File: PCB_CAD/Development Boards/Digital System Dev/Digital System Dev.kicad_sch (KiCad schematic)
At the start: 43 parts, among them J1 STLINK, J2 FADER, J7 SPI_MASTER, SW1 RESET, U1 STM32G474VETx, X1 HSE_24

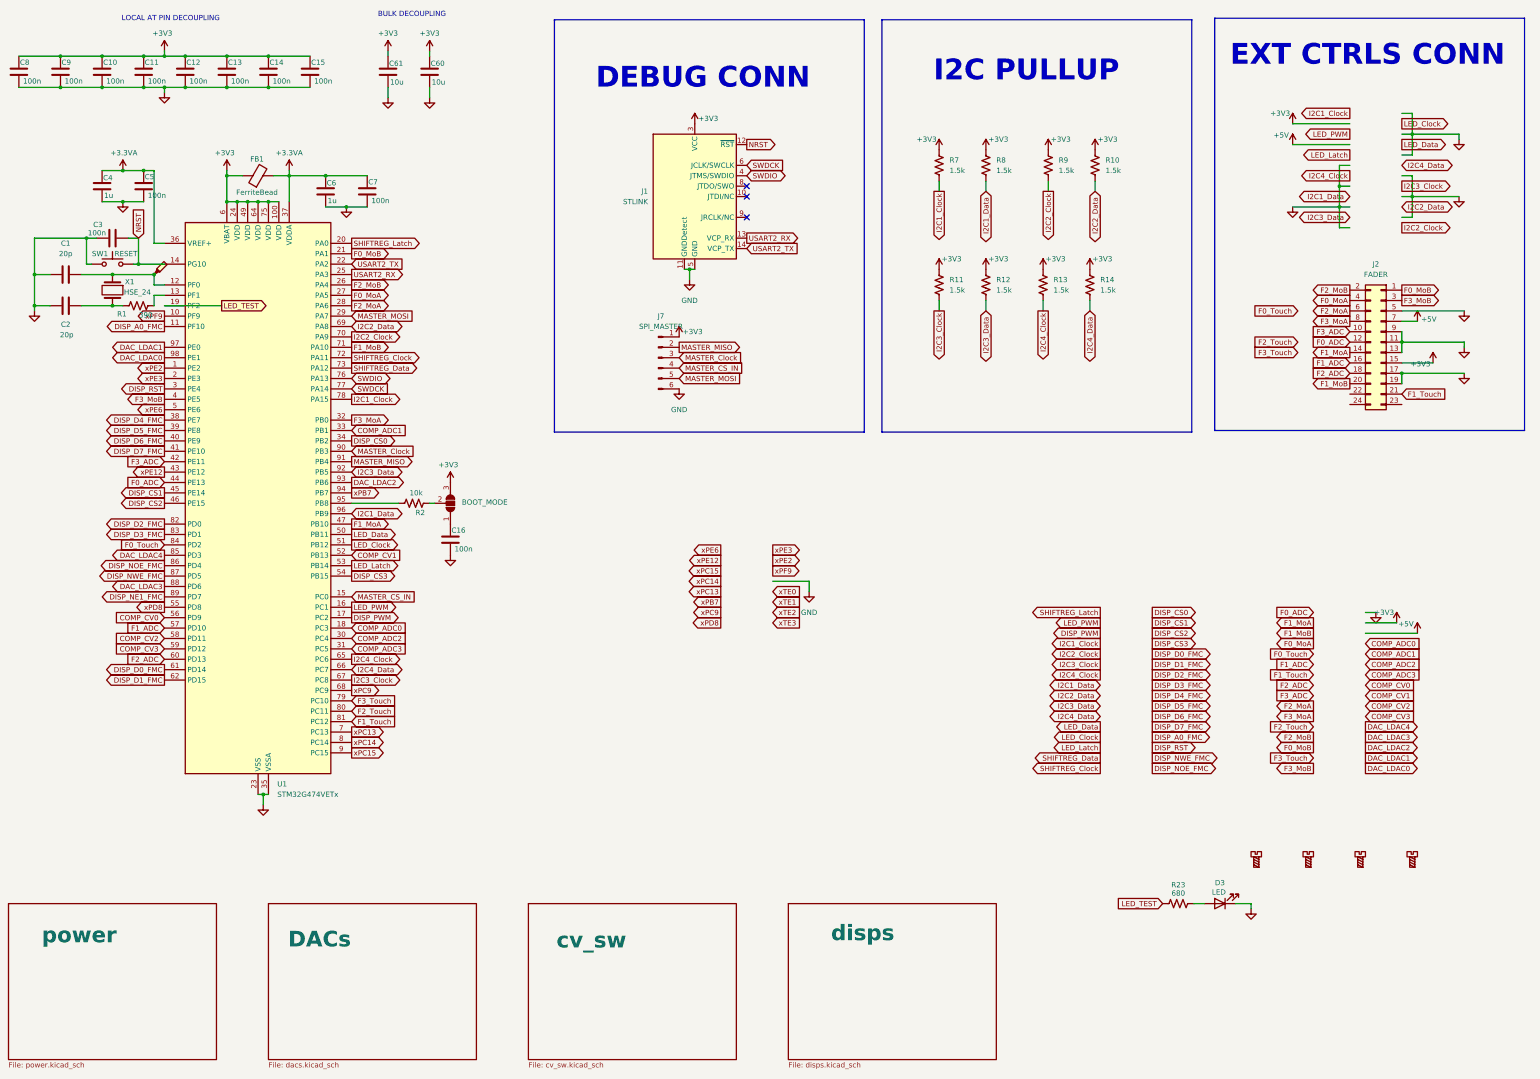
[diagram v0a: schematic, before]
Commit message: digital dev (or maybe final) board
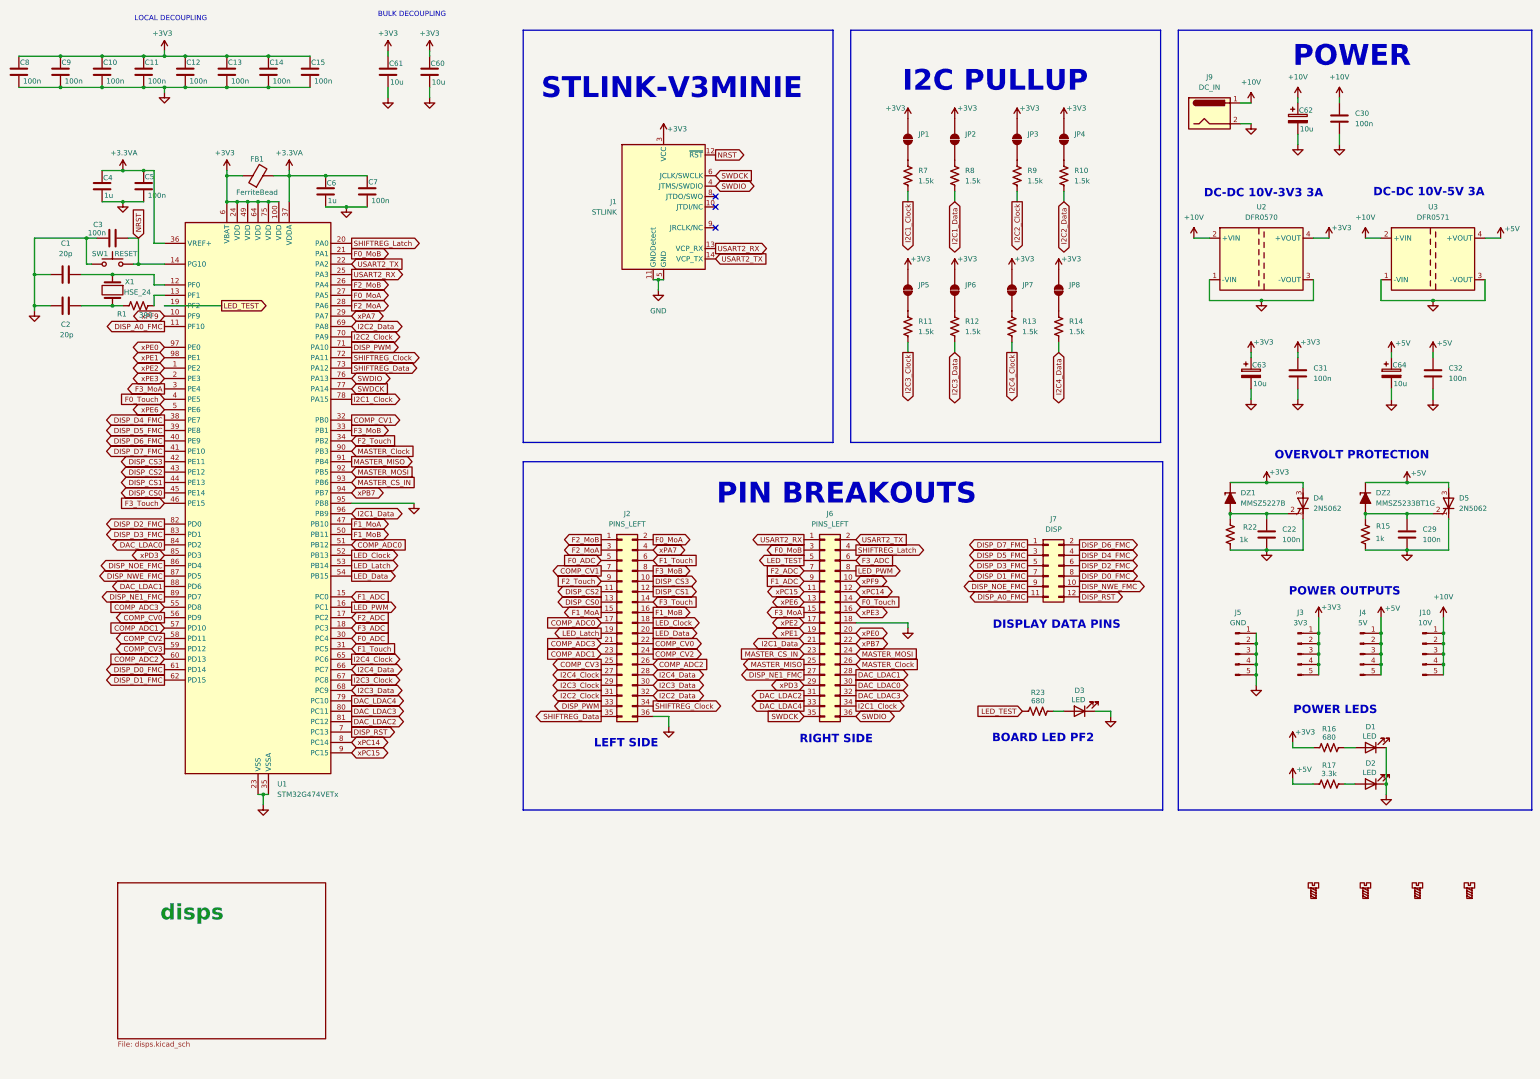
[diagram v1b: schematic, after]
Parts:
- removed C16: 100n, Capacitor_SMD:C_0603_1608Metric, symbol Device:C
- removed J2: FADER, Connector_PinHeader_1.27mm:PinHeader_2x12_P1.27mm_Vertical, symbol Connector_Generic:Conn_02x12_Odd_Even
- removed J7: SPI_MASTER, Connector_PinHeader_2.54mm:PinHeader_1x06_P2.54mm_Vertical, symbol Connector:Conn_01x06_Pin
- removed R2: 10k, Resistor_SMD:R_0603_1608Metric, symbol Device:R_US
- removed SP1: BOOT_MODE, Jumper:SolderJumper-3_P2.0mm_Open_TrianglePad1.0x1.5mm, symbol Jumper:SolderJumper_3_Open
- removed TP11: TestPoint_Probe, TestPoint:TestPoint_Keystone_5019_Miniature, symbol Connector:TestPoint_Probe
- added C22, C29, C30, C31, C32: 100n, Capacitor_SMD:C_0603_1608Metric, symbol Device:C
- added C62, C63, C64: 10u, Capacitor_SMD:CP_Elec_6.3x5.8, symbol Device:C_Polarized
- added D1, D2: LED, LED_SMD:LED_0603_1608Metric, symbol Device:LED
- added D4, D5: 2N5062, Package_TO_SOT_THT:TO-92, symbol Device:Q_SCR_KGA
- added DZ1: MMSZ5227B, Diode_SMD:D_SOD-123, symbol PCM_Diode_Zener_AKL:D_Zener_Generic
- added DZ2: MMSZ5233BT1G, Diode_SMD:D_SOD-123, symbol PCM_Diode_Zener_AKL:D_Zener_Generic
- added J10: 10V, Connector_PinSocket_2.54mm:PinSocket_1x05_P2.54mm_Vertical, symbol Connector:Conn_01x05_Pin
- added J2, J6: PINS_LEFT, Connector_PinHeader_2.54mm:PinHeader_2x18_P2.54mm_Vertical, symbol Connector_Generic:Conn_02x18_Odd_Even
- added J3: 3V3, Connector_PinSocket_2.54mm:PinSocket_1x05_P2.54mm_Vertical, symbol Connector:Conn_01x05_Pin
- added J4: 5V, Connector_PinSocket_2.54mm:PinSocket_1x05_P2.54mm_Vertical, symbol Connector:Conn_01x05_Pin
- added J5: GND, Connector_PinSocket_2.54mm:PinSocket_1x05_P2.54mm_Vertical, symbol Connector:Conn_01x05_Pin
- added J7: DISP, Connector_PinHeader_2.54mm:PinHeader_2x06_P2.54mm_Vertical, symbol Connector_Generic:Conn_02x06_Odd_Even
- added J9: DC_IN, Connector_BarrelJack:BarrelJack_Horizontal, symbol Connector:Barrel_Jack
- added JP1, JP2, JP3, JP4, JP5, JP6, JP7, JP8: SolderJumper_2_Open, Jumper:SolderJumper-2_P1.3mm_Open_TrianglePad1.0x1.5mm, symbol Jumper:SolderJumper_2_Open
- added R15, R22: 1k, Resistor_SMD:R_0603_1608Metric, symbol Device:R_US
- added R16: 680, Resistor_SMD:R_0603_1608Metric, symbol Device:R_US
- added R17: 3.3k, Resistor_SMD:R_0603_1608Metric, symbol Device:R_US
- added U2: DFR0570, My Footprints:DFR05xx_DC-DC, symbol Regulator_Switching:CRE1S0305S3C
- added U3: DFR0571, My Footprints:DFR05xx_DC-DC, symbol Regulator_Switching:CRE1S0305S3C
- H1, H2, H3, H4: LCSC (none) -> DNP
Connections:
- net xPC13 is gone; now on net DISP_RST: U1.7 (PC13)
- net xPC9 is gone; now on net I2C3_Data: U1.68 (PC9)
- net xPD8 is gone; now on net COMP_ADC3: U1.55 (PD8)
- net xPE12 is gone; now on net DISP_CS2: U1.43 (PE12)
- net +3V3: now also C31.1, C63.1, D4.3 (A), DZ1.1 (K), J3.1 (Pin_1), J3.2 (Pin_2), J3.3 (Pin_3), J3.4 (Pin_4), J3.5 (Pin_5), JP1.2 (B), JP2.2 (B), JP3.2 (B), JP4.2 (B), JP5.2 (B), JP6.2 (B), JP7.2 (B), JP8.2 (B), R16.1, U2.4 (+VOUT); no longer R10.1, R11.1, R12.1, R13.1, R14.1, R7.1, R8.1, R9.1
- net +5V: now also C32.1, C64.1, D5.3 (A), DZ2.1 (K), J4.1 (Pin_1), J4.2 (Pin_2), J4.3 (Pin_3), J4.4 (Pin_4), J4.5 (Pin_5), R17.1, U3.4 (+VOUT)
- net COMP_ADC0: now also U1.51 (PB12), J2.17 (Pin_17); no longer U1.18 (PC3)
- net COMP_ADC1: now also U1.57 (PD10), J2.23 (Pin_23); no longer U1.33 (PB1)
- net COMP_ADC2: now also U1.60 (PD13), J2.26 (Pin_26); no longer U1.30 (PC4)
- net COMP_ADC3: now also J2.21 (Pin_21); no longer U1.31 (PC5)
- net COMP_CV0: now also J2.22 (Pin_22)
- net COMP_CV1: now also U1.32 (PB0), J2.7 (Pin_7); no longer U1.52 (PB13)
- net COMP_CV2: now also J2.24 (Pin_24)
- net COMP_CV3: now also J2.25 (Pin_25)
- net DAC_LDAC0: now also U1.84 (PD2), J6.30 (Pin_30); no longer U1.98 (PE1)
- net DAC_LDAC1: now also U1.88 (PD6), J6.28 (Pin_28); no longer U1.97 (PE0)
- net DAC_LDAC2: now also U1.81 (PC12), J6.31 (Pin_31); no longer U1.93 (PB6)
- net DAC_LDAC3: now also U1.80 (PC11), J6.32 (Pin_32); no longer U1.88 (PD6)
- net DAC_LDAC4: now also U1.79 (PC10), J6.33 (Pin_33); no longer U1.85 (PD3)
- net DISP_A0_FMC: now also J7.11 (Pin_11)
- net DISP_CS0: now also U1.45 (PE14), J2.13 (Pin_13); no longer U1.34 (PB2)
- net DISP_CS1: now also U1.44 (PE13), J2.12 (Pin_12); no longer U1.45 (PE14)
- net DISP_CS2: now also J2.11 (Pin_11); no longer U1.46 (PE15)
- net DISP_CS3: now also U1.42 (PE11), J2.10 (Pin_10); no longer U1.54 (PB15)
- net DISP_D0_FMC: now also J7.8 (Pin_8)
- net DISP_D1_FMC: now also J7.7 (Pin_7)
- net DISP_D2_FMC: now also J7.6 (Pin_6)
- net DISP_D3_FMC: now also J7.5 (Pin_5)
- net DISP_D4_FMC: now also J7.4 (Pin_4)
- net DISP_D5_FMC: now also J7.3 (Pin_3)
- net DISP_D6_FMC: now also J7.2 (Pin_2)
- net DISP_D7_FMC: now also J7.1 (Pin_1)
- net DISP_NE1_FMC: now also J6.27 (Pin_27)
- net DISP_NOE_FMC: now also J7.9 (Pin_9)
- net DISP_NWE_FMC: now also J7.10 (Pin_10)
- net DISP_PWM: now also U1.71 (PA10), J2.33 (Pin_33); no longer U1.17 (PC2)
- net DISP_RST: now also J7.12 (Pin_12); no longer U1.3 (PE4)
- net F0_ADC: now also U1.30 (PC4), J2.5 (Pin_5); no longer U1.44 (PE13)
- net F0_MoA: now also J2.2 (Pin_2)
- net F0_MoB: now also J6.3 (Pin_3)
- net F0_Touch: now also U1.4 (PE5), J6.14 (Pin_14); no longer U1.84 (PD2)
- net F1_ADC: now also U1.15 (PC0), J6.9 (Pin_9); no longer U1.57 (PD10)
- net F1_MoA: now also J2.15 (Pin_15)
- net F1_MoB: now also U1.50 (PB11), J2.16 (Pin_16); no longer U1.71 (PA10)
- net F1_Touch: now also U1.31 (PC5), J2.6 (Pin_6); no longer U1.81 (PC12)
- net F2_ADC: now also U1.17 (PC2), J6.7 (Pin_7); no longer U1.60 (PD13)
- net F2_MoA: now also J2.3 (Pin_3)
- net F2_MoB: now also J2.1 (Pin_1)
- net F2_Touch: now also U1.34 (PB2), J2.9 (Pin_9); no longer U1.80 (PC11)
- net F3_ADC: now also U1.18 (PC3), J6.6 (Pin_6); no longer U1.42 (PE11)
- net F3_MoA: now also U1.3 (PE4), J6.15 (Pin_15); no longer U1.32 (PB0)
- net F3_MoB: now also U1.33 (PB1), J2.8 (Pin_8); no longer U1.4 (PE5)
- net F3_Touch: now also U1.46 (PE15), J2.14 (Pin_14); no longer U1.79 (PC10)
- net GND: now also U1.95 (PB8), C22.2, C29.2, C30.2, C31.2, C32.2, C62.2, C63.2, C64.2, D1.1 (K), D2.1 (K), D4.1 (K), D5.1 (K), J2.36 (Pin_36), J5.1 (Pin_1), J5.2 (Pin_2), J5.3 (Pin_3), J5.4 (Pin_4), J5.5 (Pin_5), J6.18 (Pin_18), J9.2, R15.1, R22.1, U2.1 (-VIN), U2.3 (-VOUT), U3.1 (-VIN), U3.3 (-VOUT)
- net I2C1_Clock: now also J6.34 (Pin_34)
- net I2C1_Data: now also J6.21 (Pin_21)
- net I2C2_Clock: now also J2.31 (Pin_31)
- net I2C2_Data: now also J2.32 (Pin_32)
- net I2C3_Clock: now also J2.29 (Pin_29)
- net I2C3_Data: now also J2.30 (Pin_30); no longer U1.92 (PB5)
- net I2C4_Clock: now also J2.27 (Pin_27)
- net I2C4_Data: now also J2.28 (Pin_28)
- net LED_Clock: now also U1.52 (PB13), J2.18 (Pin_18); no longer U1.51 (PB12)
- net LED_Data: now also U1.54 (PB15), J2.20 (Pin_20); no longer U1.50 (PB11)
- net LED_Latch: now also J2.19 (Pin_19)
- net LED_PWM: now also J6.8 (Pin_8)
- net LED_TEST: now also J6.5 (Pin_5)
- net MASTER_CS_IN: now also U1.93 (PB6), J6.23 (Pin_23); no longer U1.15 (PC0)
- net MASTER_Clock: now also J6.26 (Pin_26)
- net MASTER_MISO: now also J6.25 (Pin_25)
- net MASTER_MOSI: now also U1.92 (PB5), J6.24 (Pin_24); no longer U1.29 (PA7)
- net SHIFTREG_Clock: now also J2.34 (Pin_34)
- net SHIFTREG_Data: now also J2.35 (Pin_35)
- net SHIFTREG_Latch: now also J6.4 (Pin_4)
- net SWDCK: now also J6.35 (Pin_35)
- net SWDIO: now also J6.36 (Pin_36)
- net USART2_RX: now also J6.1 (Pin_1)
- net USART2_TX: now also J6.2 (Pin_2)
- net xPB7: now also J6.22 (Pin_22)
- net xPC14: now also J6.12 (Pin_12)
- net xPC15: now also J6.11 (Pin_11)
- net xPE2: now also J6.17 (Pin_17)
- net xPE3: now also J6.16 (Pin_16)
- net xPE6: now also J6.13 (Pin_13)
- net xPF9: now also J6.10 (Pin_10)
- new net: JP1.1 (A), R7.1
- new net: JP7.1 (A), R13.1
- new net: JP6.1 (A), R12.1
- new net: JP2.1 (A), R8.1
- new net: JP4.1 (A), R10.1
- new net: JP3.1 (A), R9.1
- new net: JP5.1 (A), R11.1
- new net: C29.1, D5.2 (G), DZ2.2 (A), R15.2
- new net: D1.2 (A), R16.2
- new net: C22.1, D4.2 (G), DZ1.2 (A), R22.2
- new net: JP8.1 (A), R14.1
- new net: D2.2 (A), R17.2
- new net +10V: C30.1, C62.1, J10.1 (Pin_1), J10.2 (Pin_2), J10.3 (Pin_3), J10.4 (Pin_4), J10.5 (Pin_5), J9.1, U2.2 (+VIN), U3.2 (+VIN)
- new net xPA7: J2.4 (Pin_4), U1.29 (PA7)
- new net xPD3: J6.29 (Pin_29), U1.85 (PD3)
- new net xPE0: J6.20 (Pin_20), U1.97 (PE0)
- new net xPE1: J6.19 (Pin_19), U1.98 (PE1)
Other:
- removed sheet DACs
- removed sheet cv_sw
- removed sheet power
- note added: "BOARD LED PF2"
- note added: "DC-DC 10V-3V3 3A"
- note added: "DC-DC 10V-5V 3A"
- note added: "DISPLAY DATA PINS"
- note added: "LEFT SIDE"
- note added: "LOCAL DECOUPLING"
- note added: "OVERVOLT PROTECTION"
- note added: "PIN BREAKOUTS"
- note added: "POWER"
- note added: "POWER LEDS"
- note added: "POWER OUTPUTS"
- note added: "RIGHT SIDE"
- note added: "STLINK-V3MINIE"
- note removed: "DEBUG CONN"
- note removed: "EXT CTRLS CONN"
- note removed: "LOCAL AT PIN DECOUPLING"
- moved on the sheet: D3, J1, R10, R11, R12, R13, R14, R23, R7, R8, R9
